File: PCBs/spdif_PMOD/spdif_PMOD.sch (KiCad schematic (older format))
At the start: 11 parts, among them J1 Conn_01x06_Male, J2 Conn_01x04_Male, J3 Conn_Coaxial, U1 74HC04

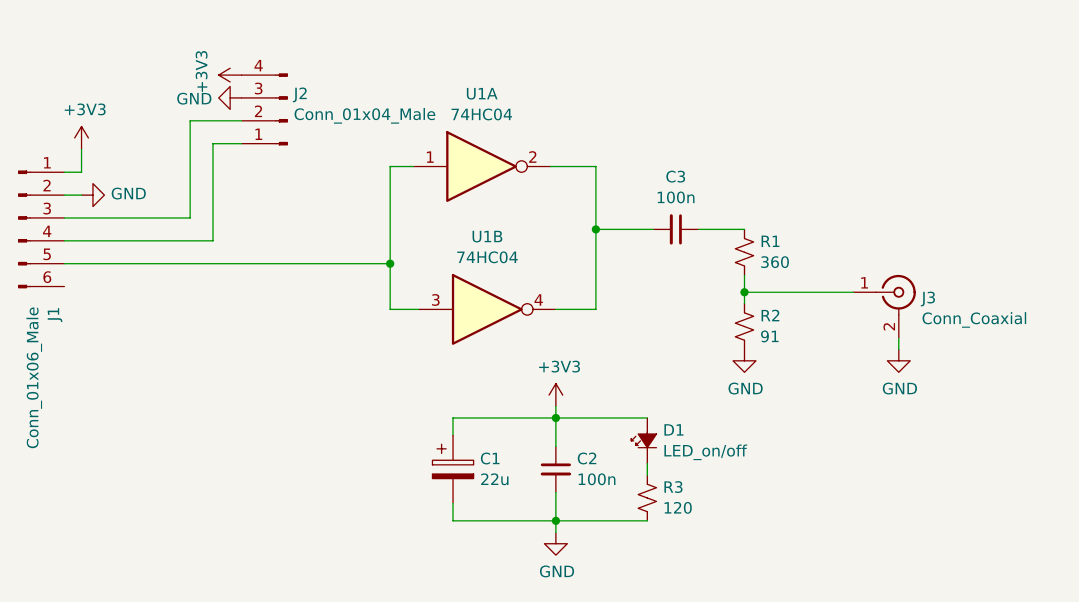
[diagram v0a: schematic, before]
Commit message: agrego PCB spdif_pmod terminado
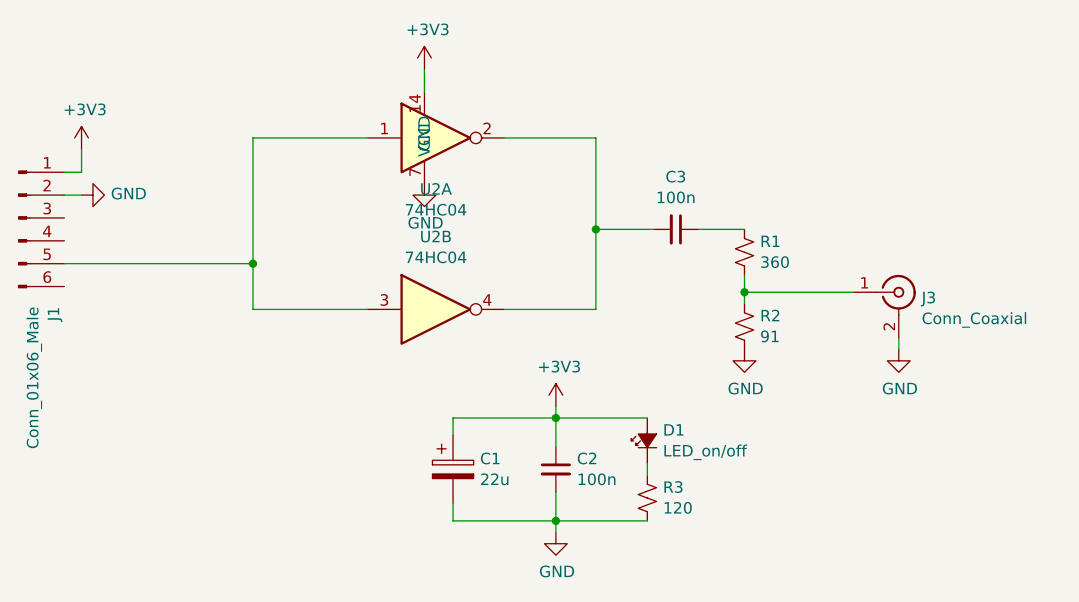
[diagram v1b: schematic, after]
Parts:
- removed J2: Conn_01x04_Male, Connector_PinHeader_2.54mm:PinHeader_1x04_P2.54mm_Vertical, symbol Connector:Conn_01x04_Male
- removed U1: 74HC04, Package_DIP:DIP-14_W7.62mm_LongPads, symbol 74xx:74HC04
- added U2: 74HC04, Package_DIP:DIP-14_W7.62mm_LongPads, symbol spdif_PMOD-rescue:74HC04-74xxMAXIM
- J3: footprint Connector_Coaxial:BNC_PanelMountable_Vertical -> Connector_BarrelJack:BarrelJack_CUI_PJ-063AH_Horizontal
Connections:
- net +3V3: now also U2.14 (VCC)
- net GND: now also U2.7 (GND)
- net at J1.5 (Pin_5): now also U2.1, U2.3
- net at C3.2: now also U2.2, U2.4
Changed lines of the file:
@@
 $EndDescr
-$Comp
-L 74xx:74HC04 U1
-U 1 1 5DC5747B
-P 5900 2975
-F 0 "U1" H 5900 3292 50  0000 C CNN
-F 1 "74HC04" H 5900 3201 50  0000 C CNN
-F 2 "Package_DIP:DIP-14_W7.62mm_LongPads" H 5900 2975 50  0001 C CNN
-F 3 "https://assets.nexperia.com/documents/data-sheet/74HC_HCT04.pdf" H 5900 2975 50  0001 C CNN
-	1    5900 2975
-	1    0    0    -1
-$EndComp
-$Comp
-L 74xx:74HC04 U1
-U 2 1 5DC57742
-P 5925 3600
-F 0 "U1" H 5925 3917 50  0000 C CNN
-F 1 "74HC04" H 5925 3826 50  0000 C CNN
-F 2 "Package_DIP:DIP-14_W7.62mm_LongPads" H 5925 3600 50  0001 C CNN
-F 3 "https://assets.nexperia.com/documents/data-sheet/74HC_HCT04.pdf" H 5925 3600 50  0001 C CNN
-	2    5925 3600
-	1    0    0    -1
-$EndComp
-Wire Wire Line
-	5600 2975 5500 2975
-Wire Wire Line
-	5500 3600 5625 3600
-Wire Wire Line
-	6200 2975 6400 2975
-Wire Wire Line
-	6225 3600 6400 3600
 $Comp
 L Device:C_Small C3
@@
 Wire Wire Line
 	6650 3250 6400 3250
-Wire Wire Line
-	6400 2975 6400 3250
-Connection ~ 6400 3250
-Wire Wire Line
-	6400 3250 6400 3600
 $Comp
 L Device:R_Small_US R1
@@
 F 0 "J3" H 7825 3500 50  0000 L CNN
 F 1 "Conn_Coaxial" H 7825 3409 50  0000 L CNN
-F 2 "Connector_Coaxial:BNC_PanelMountable_Vertical" H 7725 3525 50  0001 C CNN
+F 2 "Connector_BarrelJack:BarrelJack_CUI_PJ-063AH_Horizontal" H 7725 3525 50  0001 C CNN
 F 3 " ~" H 7725 3525 50  0001 C CNN
 	1    7725 3525
@@
 	1    0    0    -1
 $EndComp
-$Comp
-L Connector:Conn_01x04_Male J2
-U 1 1 5DC6EA21
-P 5050 2775
-F 0 "J2" H 5022 2657 50  0000 R CNN
-F 1 "Conn_01x04_Male" H 5022 2748 50  0000 R CNN
-F 2 "Connector_PinHeader_2.54mm:PinHeader_1x04_P2.54mm_Vertical" H 5050 2775 50  0001 C CNN
-F 3 "~" H 5050 2775 50  0001 C CNN
-	1    5050 2775
-	-1   0    0    1
-$EndComp
-Wire Wire Line
-	5500 2975 5500 3400
-Wire Wire Line
-	4075 3400 5500 3400
-Connection ~ 5500 3400
-Wire Wire Line
-	5500 3400 5500 3600
+Wire Wire Line
+	4075 3400 4900 3400
 Wire Wire Line
 	4150 3100 4075 3100
-Wire Wire Line
-	4075 3200 4625 3200
-Wire Wire Line
-	4625 3200 4625 2775
-Wire Wire Line
-	4625 2775 4850 2775
-Wire Wire Line
-	4075 3300 4725 3300
-Wire Wire Line
-	4725 3300 4725 2875
-Wire Wire Line
-	4725 2875 4850 2875
-$Comp
-L power:GND #PWR0107
-U 1 1 5DC78301
-P 4850 2675
-F 0 "#PWR0107" H 4850 2425 50  0001 C CNN
-F 1 "GND" V 4855 2547 50  0000 R CNN
-F 2 "" H 4850 2675 50  0001 C CNN
-F 3 "" H 4850 2675 50  0001 C CNN
-	1    4850 2675
-	0    1    1    0
-$EndComp
 $Comp
 L Device:R_Small_US R3
@@
 	6225 4525 6625 4525
 $Comp
-L power:+3V3 #PWR?
+L power:+3V3 #PWR0103
 U 1 1 5DC9B2DF
 P 4150 2900
-F 0 "#PWR?" H 4150 2750 50  0001 C CNN
+F 0 "#PWR0103" H 4150 2750 50  0001 C CNN
 F 1 "+3V3" H 4165 3073 50  0000 C CNN
 F 2 "" H 4150 2900 50  0001 C CNN
@@
 $EndComp
 $Comp
-L power:+3V3 #PWR?
-U 1 1 5DC9D5F2
-P 4850 2575
-F 0 "#PWR?" H 4850 2425 50  0001 C CNN
-F 1 "+3V3" H 4865 2748 50  0000 C CNN
-F 2 "" H 4850 2575 50  0001 C CNN
-F 3 "" H 4850 2575 50  0001 C CNN
-	1    4850 2575
-	0    -1   -1   0
-$EndComp
-$Comp
-L power:+3V3 #PWR?
+L power:+3V3 #PWR0106
 U 1 1 5DC9F6C0
 P 6225 4025
-F 0 "#PWR?" H 6225 3875 50  0001 C CNN
+F 0 "#PWR0106" H 6225 3875 50  0001 C CNN
 F 1 "+3V3" H 6240 4198 50  0000 C CNN
 F 2 "" H 6225 4025 50  0001 C CNN
@@
 	1    0    0    -1
 $EndComp
+$Comp
+L spdif_PMOD-rescue:74HC04-74xxMAXIM U2
+U 1 1 5DC799D4
+P 5700 2850
+F 0 "U2" H 5700 2625 50  0000 C CNN
+F 1 "74HC04" H 5700 2534 50  0000 C CNN
+F 2 "Package_DIP:DIP-14_W7.62mm_LongPads" H 5700 2850 50  0001 C CNN
+F 3 "https://assets.nexperia.com/documents/data-sheet/74HC_HCT04.pdf" H 5700 2850 50  0001 C CNN
+	1    5700 2850
+	1    0    0    -1
+$EndComp
+Wire Wire Line
+	5400 2850 4900 2850
+Wire Wire Line
+	4900 2850 4900 3400
+Wire Wire Line
+	6400 2850 6000 2850
+Wire Wire Line
+	6400 2850 6400 3250
+$Comp
+L spdif_PMOD-rescue:74HC04-74xxMAXIM U2
+U 2 1 5DC8678B
+P 5700 3600
+F 0 "U2" H 5700 3917 50  0000 C CNN
+F 1 "74HC04" H 5700 3826 50  0000 C CNN
+F 2 "Package_DIP:DIP-14_W7.62mm_LongPads" H 5700 3600 50  0001 C CNN
+F 3 "https://assets.nexperia.com/documents/data-sheet/74HC_HCT04.pdf" H 5700 3600 50  0001 C CNN
+	2    5700 3600
+	1    0    0    -1
+$EndComp
+Wire Wire Line
+	5400 3600 4900 3600
+Wire Wire Line
+	4900 3600 4900 3400
+Connection ~ 4900 3400
+Wire Wire Line
+	6000 3600 6400 3600
+Wire Wire Line
+	6400 3600 6400 3250
+Connection ~ 6400 3250
+Wire Wire Line
+	5650 2550 5650 2650
+$Comp
+L power:+3V3 #PWR0107
+U 1 1 5DC89E2F
+P 5650 2550
+F 0 "#PWR0107" H 5650 2400 50  0001 C CNN
+F 1 "+3V3" H 5665 2723 50  0000 C CNN
+F 2 "" H 5650 2550 50  0001 C CNN
+F 3 "" H 5650 2550 50  0001 C CNN
+	1    5650 2550
+	1    0    0    -1
+$EndComp
+$Comp
+L power:GND #PWR0108
+U 1 1 5DC91D1E
+P 5650 3050
+F 0 "#PWR0108" H 5650 2800 50  0001 C CNN
+F 1 "GND" H 5655 2877 50  0000 C CNN
+F 2 "" H 5650 3050 50  0001 C CNN
+F 3 "" H 5650 3050 50  0001 C CNN
+	1    5650 3050
+	1    0    0    -1
+$EndComp
